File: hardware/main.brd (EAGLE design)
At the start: 160 x 100 mm, 38 parts, among them IC1 FT232RL, J1 POWER_JACKPTH_BREAD, M1 SERVO, M2 SERVO, M3 SERVO, P1 61729-1011BLF, X1 STEREOJACK

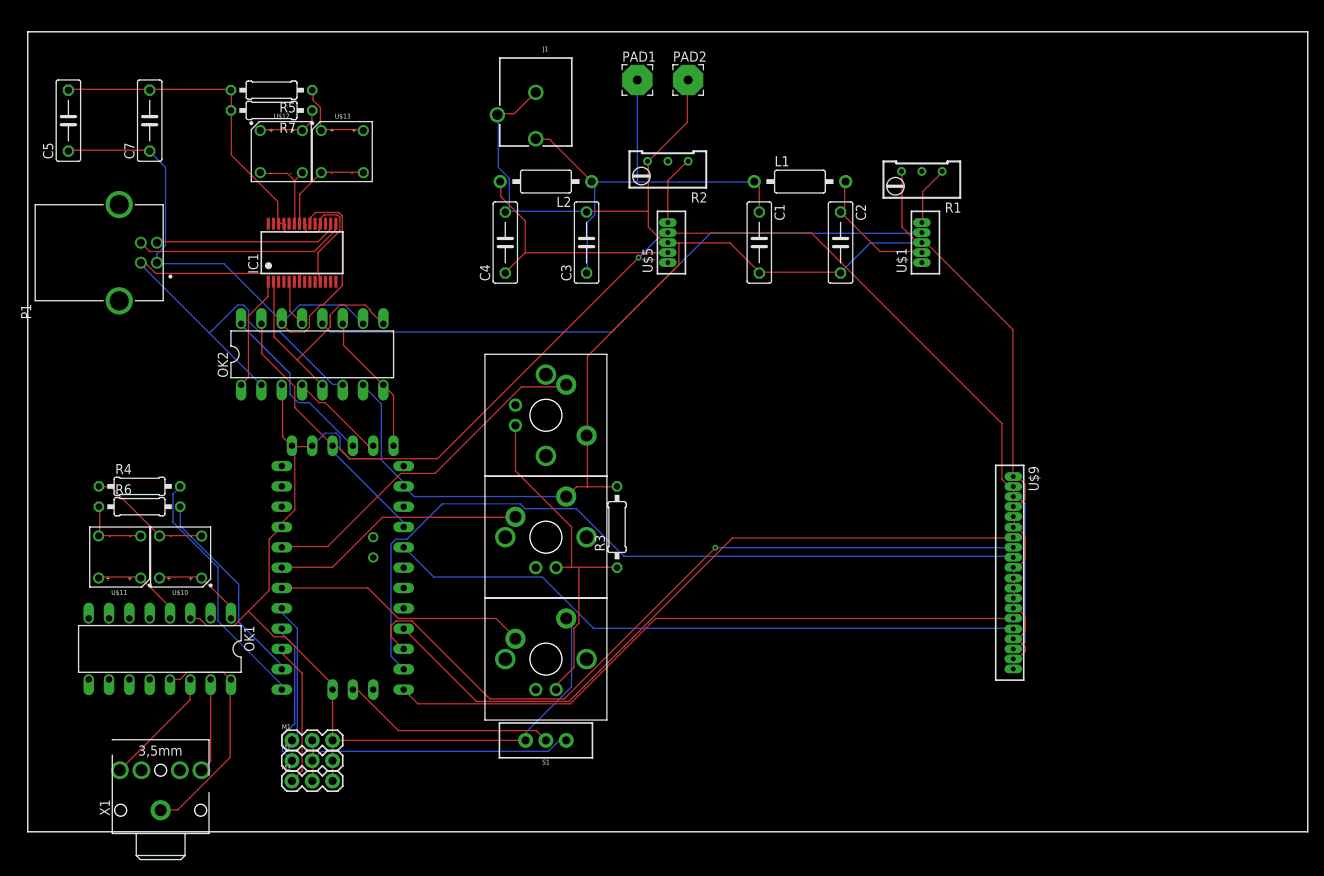
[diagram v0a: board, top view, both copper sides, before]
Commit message: Updated hardware files for eagle
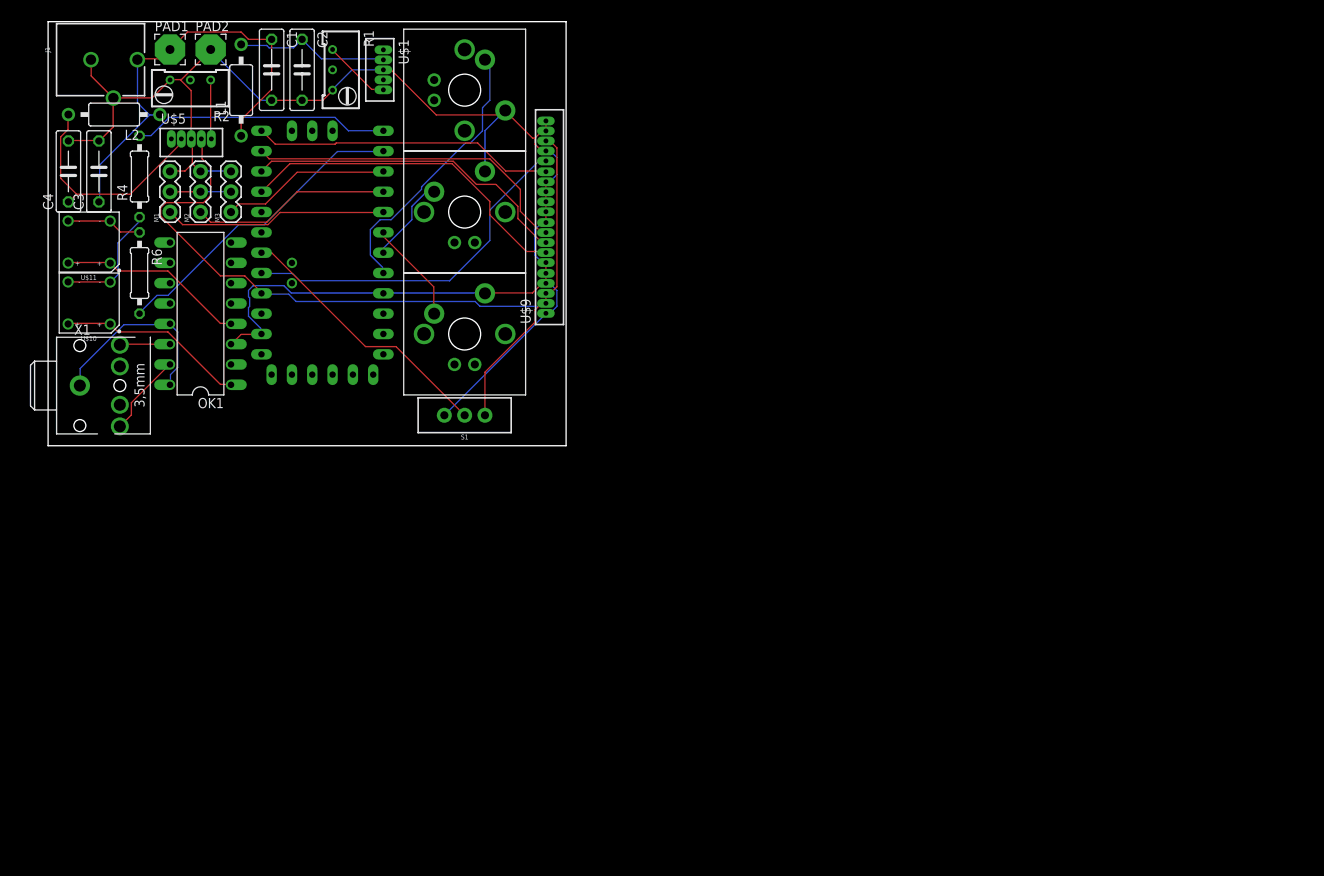
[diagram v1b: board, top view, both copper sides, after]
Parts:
- removed C5: 10µF, rcl:C075-032X103
- removed C7: 0.1µF, rcl:C075-032X103
- removed IC1: FT232RL, ftdichip:SSOP28
- removed OK2: ILQ1, optocoupler:DIL16
- removed P1: 61729-1011BLF, Common-Parts-Library-Eagle:FCI_61729-1011BLF
- removed R3, R5, R7: 220Ω, rcl:0207/10
- removed U$12, U$13: PIRANHA_LED, Mel_Custom:LED_PIRANHA_5MM
- moved R1 73.7 mm to (39.4, 95.2), turned to 180 degrees
- moved M3 71.5 mm to (25.4, 77.5), turned to 90 degrees
- moved L1 70.8 mm to (26.7, 92.7), turned to 90 degrees
- moved C2 70.7 mm to (34.3, 95.2)
- moved U$1 70.7 mm to (44.5, 95.2), turned to 270 degrees
- moved M2 69.5 mm to (21.6, 77.5), turned to 90 degrees
- moved M1 67.8 mm to (17.8, 77.5), turned to 90 degrees
- moved C1 64.7 mm to (30.5, 95.2)
- moved U$9 63.7 mm to (64.8, 67.3), turned to 90 degrees
- moved J1 63.6 mm to (0.00, 96.5), turned to 270 degrees
- moved C3 61.6 mm to (8.89, 82.5)
- moved U$5 61.0 mm to (20.4, 86.6), turned to 0 degrees
- moved R2 60.5 mm to (20.3, 92.7)
- moved PAD2 59.8 mm to (22.9, 97.8)
- moved PAD1 58.5 mm to (17.8, 97.8)
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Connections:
- removed net N$20: OK2.16, U$2.RX1-1
- removed net N$28: C5.1, C7.1, IC1.20, OK2.10, OK2.14, P1.1
- removed net N$36: S1.2, U$2.A6
- removed net N$37: IC1.2, OK2.5, OK2.9
- removed net N$39: IC1.15, P1.3
- removed net N$40: IC1.16, P1.2
- removed net N$41: OK2.4, U$2.TX0-1
- removed net N$43: IC1.5, OK2.13
- removed net N$44: OK2.11, OK2.8, U$2.DTR
- removed net N$45: R5.1, U$13.+@0, U$13.+@1
- removed net N$46: R7.1, U$12.+@0, U$12.+@1
- removed net N$47: IC1.23, U$12.-@0, U$12.-@1
- removed net N$48: IC1.1, OK2.1
- removed net N$50: C5.2, C7.2, IC1.11, IC1.18, IC1.21, IC1.25, IC1.26, IC1.7, OK2.2, OK2.6, P1.4, R5.2, R7.2
- removed net N$52: IC1.22, U$13.-@0, U$13.-@1
- removed net VCCIO: IC1.4
- net N$15: now also S1.2, U$2.A1; no longer R3.1, U$6.LED2, U$7.LED2, U$8.LED2
- net N$19: no longer OK2.12
- net N$23: no longer S1.3
- net N$38: no longer OK2.3, OK2.7, R3.2, U$2.GND2, U$2.GND3, U$2.GND4
- net N$42: now also S1.3; no longer OK2.15, U$2.VCC1
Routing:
- net N$38: track 373.4 -> 206.3 mm
- net N$50: track 129.7 -> 0.00 mm
- net N$28: track 82.0 -> 0.00 mm
- net N$19: track 80.5 -> 0.00 mm
- net N$42: track 170.1 -> 108.3 mm, vias 1 -> 0
- net N$21: track 99.0 -> 41.4 mm
- net N$18: track 93.5 -> 41.2 mm, vias 1 -> 0
- net N$25: track 88.5 -> 42.7 mm
- net N$24: track 81.4 -> 37.9 mm
- net N$22: track 80.4 -> 44.4 mm
- net N$37: track 31.0 -> 0.00 mm
- net N$23: track 38.2 -> 7.62 mm
- net N$36: track 26.8 -> 0.00 mm
- net N$39: track 26.7 -> 0.00 mm
- net N$40: track 23.1 -> 0.00 mm
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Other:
- board size 160 x 100 mm -> 64.8 x 53 mm
